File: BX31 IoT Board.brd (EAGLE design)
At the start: 45 x 22.3 mm, 17 parts, among them IC1 CAT24C32 YI-GT3, Q1 BSS138, Q2 BSS138, Q3 BSS138

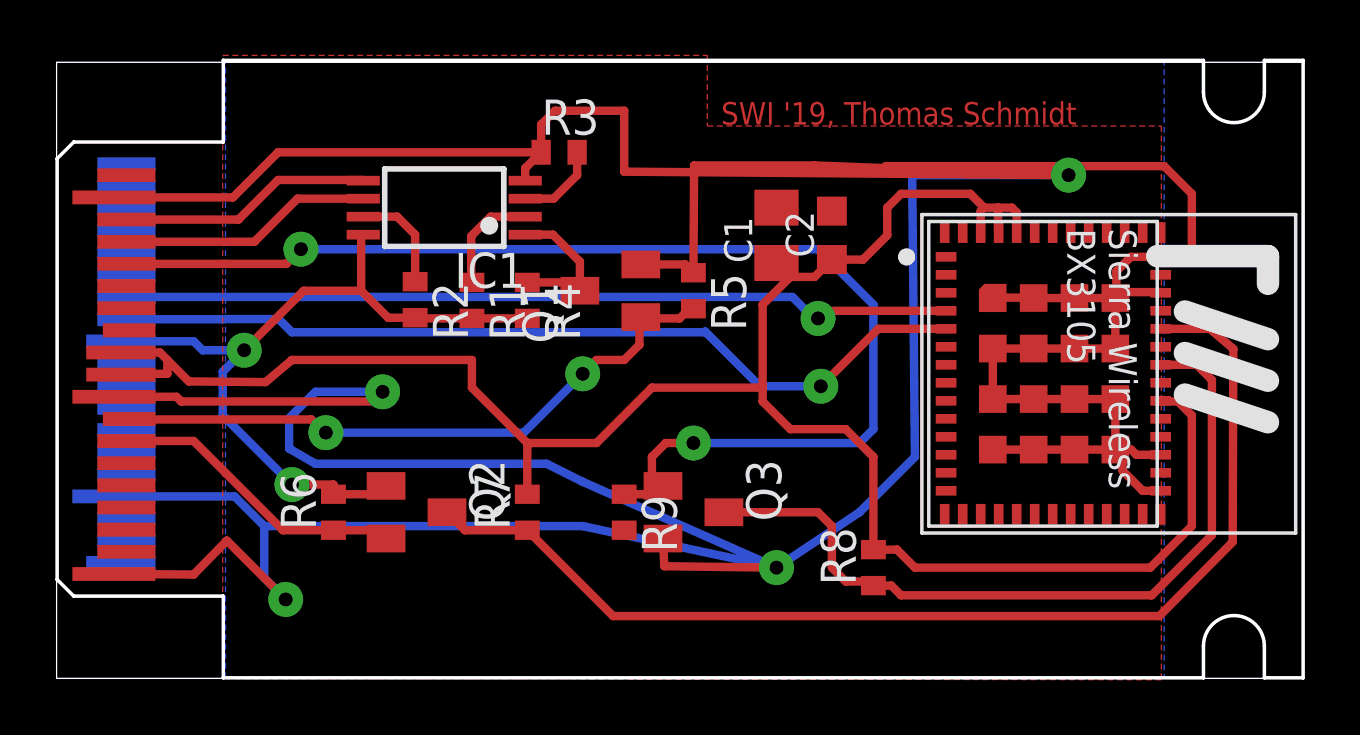
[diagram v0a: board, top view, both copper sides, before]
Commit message: removed multi
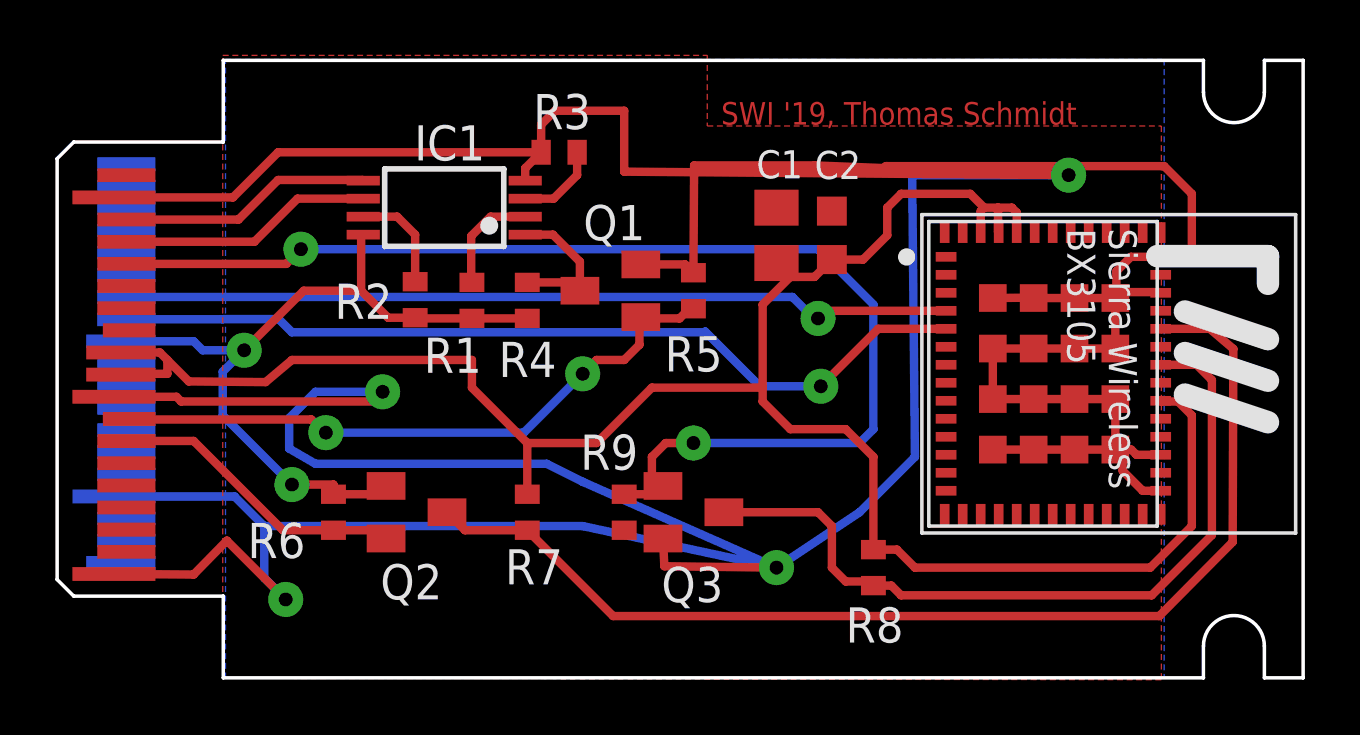
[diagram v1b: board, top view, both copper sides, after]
